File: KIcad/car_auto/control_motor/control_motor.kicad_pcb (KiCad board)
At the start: 2 copper layers, 96 x 96 mm, 8 parts, among them J1 B6P-VH_LF__SN_, J4 B2P-VH_LF__SN_, U1 YAAJ_DCDC_StepDown_LM2596, U2 L298N DUAL H-BRIDGE MOTOR DRI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

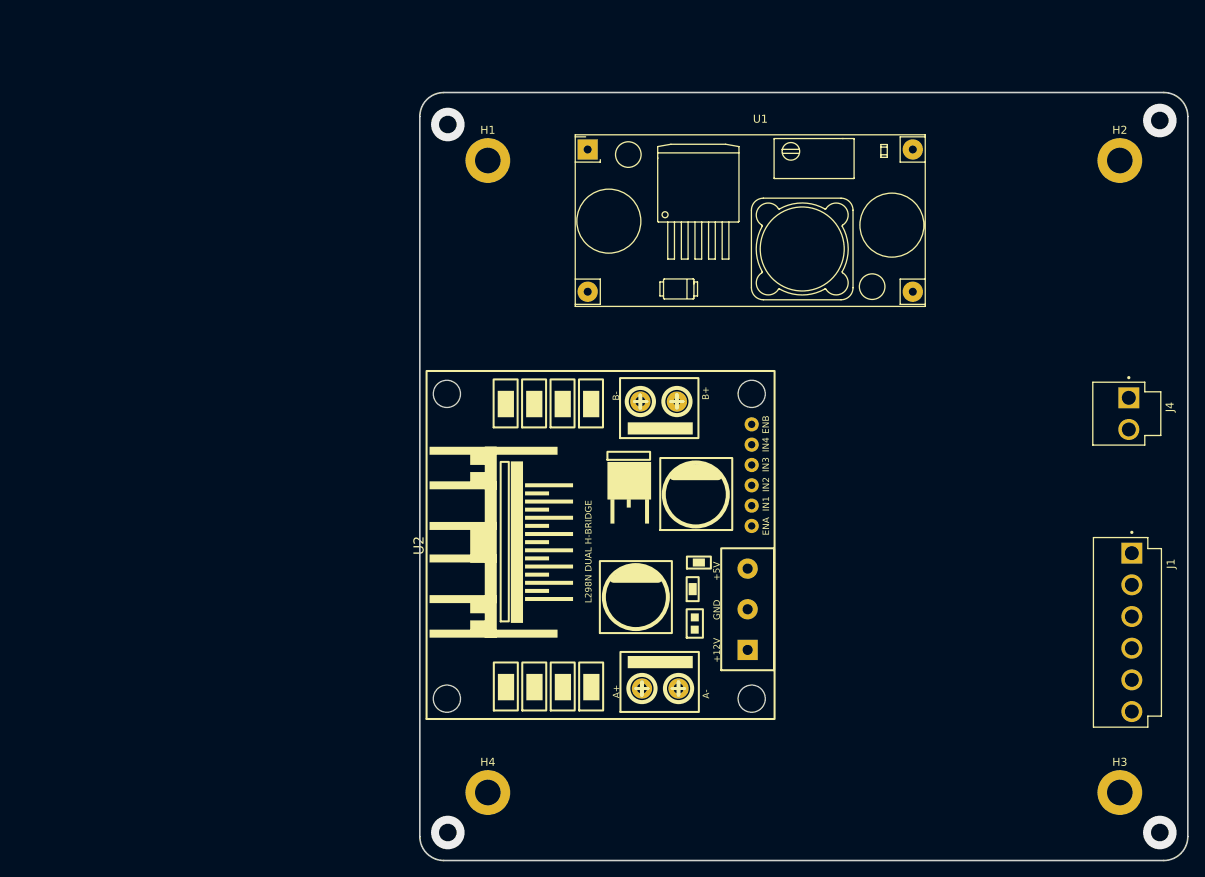
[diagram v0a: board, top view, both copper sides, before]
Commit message: feat: Implementação da classe para controle dos motores via Bluetooth.
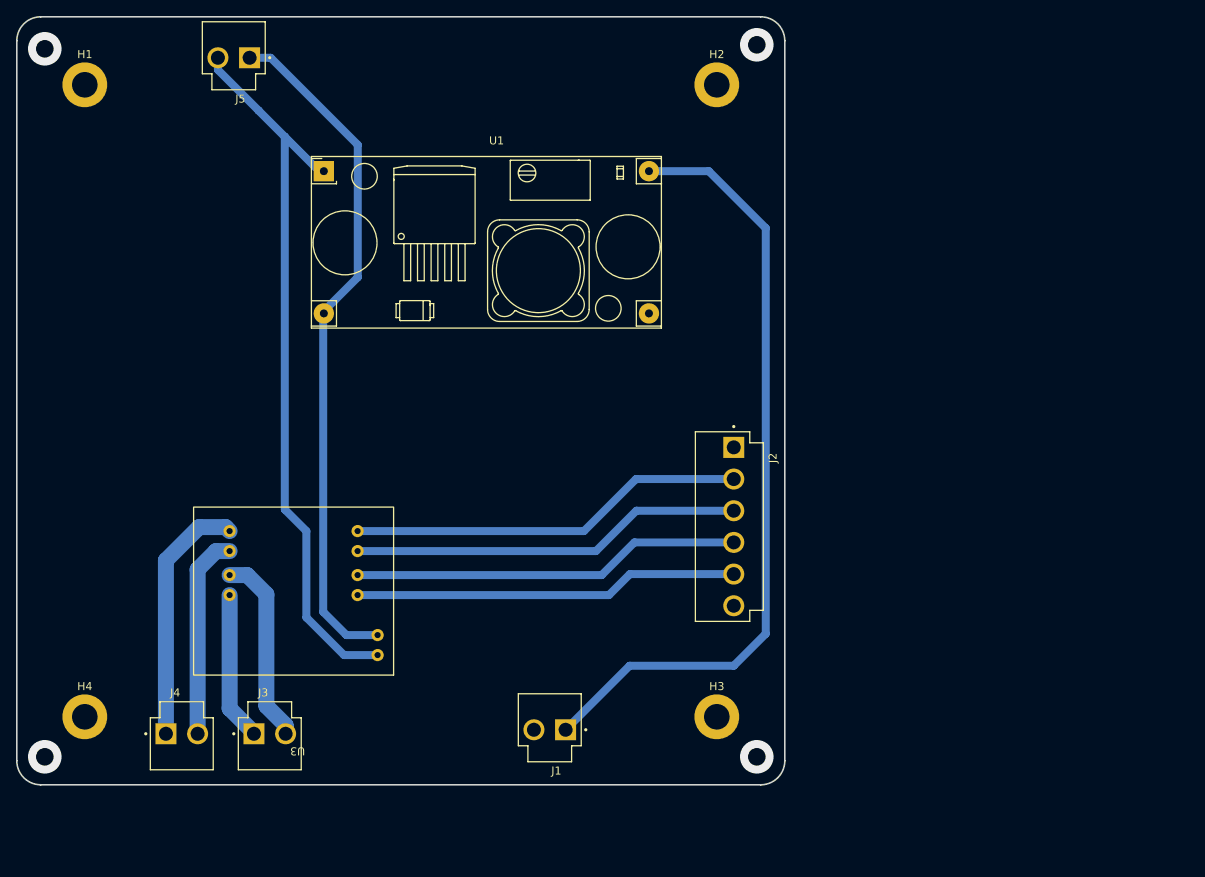
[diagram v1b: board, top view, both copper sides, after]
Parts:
- removed U2: L298N DUAL H-BRIDGE MOTOR DRIVER MODULE, importados:L298N DUAL H-BRIDGE MOTOR DRIVER MODULE FOOTPRINT
- added J2: B6P-VH_LF__SN_, importados:JST_B6P-VH_LF__SN_, F.Cu at (186.6, 109.6)
- added J3: B2P-VH_LF__SN_, importados:JST_B2P-VH_LF__SN_, F.Cu at (128.6, 135.5)
- added J5: B2P-VH_LF__SN_, importados:JST_B2P-VH_LF__SN_, F.Cu at (124.1, 51.0)
- added U3: ~, importados:Mini Driver Motor Ponte H L298n, F.Cu at (132.1, 137.2)
- J1: value B6P-VH_LF__SN_ -> B2P-VH_LF__SN_; footprint importados:JST_B6P-VH_LF__SN_ -> importados:JST_B2P-VH_LF__SN_
- moved J4 125.0 mm to (117.6, 135.5), turned to 0 degrees
- moved J1 73.8 mm to (163.6, 135.0), turned to 180 degrees
- moved H1 51.3 mm to (105.5, 54.4)
- moved H2 51.3 mm to (184.5, 54.4)
- moved H3 51.3 mm to (184.5, 133.4)
- moved H4 51.3 mm to (105.5, 133.4)
- moved U1 33.1 mm to (135.4, 65.2)
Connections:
- J1 pad 1: (no net) -> 5V
- J1 pad 2: (no net) -> GND
- J4 pad 1: (no net) -> OUT4
- J4 pad 2: (no net) -> OUT3
- U1 pad 1: unconnected-(U1-Vin-Pad1) -> 9V
- U1 pad 2: unconnected-(U1-GND-Pad2) -> GND2
- U1 pad 3: unconnected-(U1-GND-Pad3) -> GND
- U1 pad 4: unconnected-(U1-Vout-Pad4) -> 5V
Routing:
- net 5V: track 0.00 -> 98.2 mm
- net 9V: track 0.00 -> 92.1 mm
- net GND2: track 0.00 -> 86.2 mm
- net IN4-B: track 0.00 -> 49.7 mm
- net IN3-B: track 0.00 -> 49.1 mm
- net IN2-A: track 0.00 -> 48.7 mm
- net IN1-A: track 0.00 -> 48.1 mm
- net OUT4: track 0.00 -> 31.6 mm
- net OUT3: track 0.00 -> 25.5 mm
- net OUT2: track 0.00 -> 24.0 mm
- net OUT1: track 0.00 -> 18.6 mm
